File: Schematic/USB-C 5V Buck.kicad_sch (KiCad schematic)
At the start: 17 parts, among them Q25 CSD19531Q5A, Q26 CSD19531Q5A, U12 LM5148RGYR

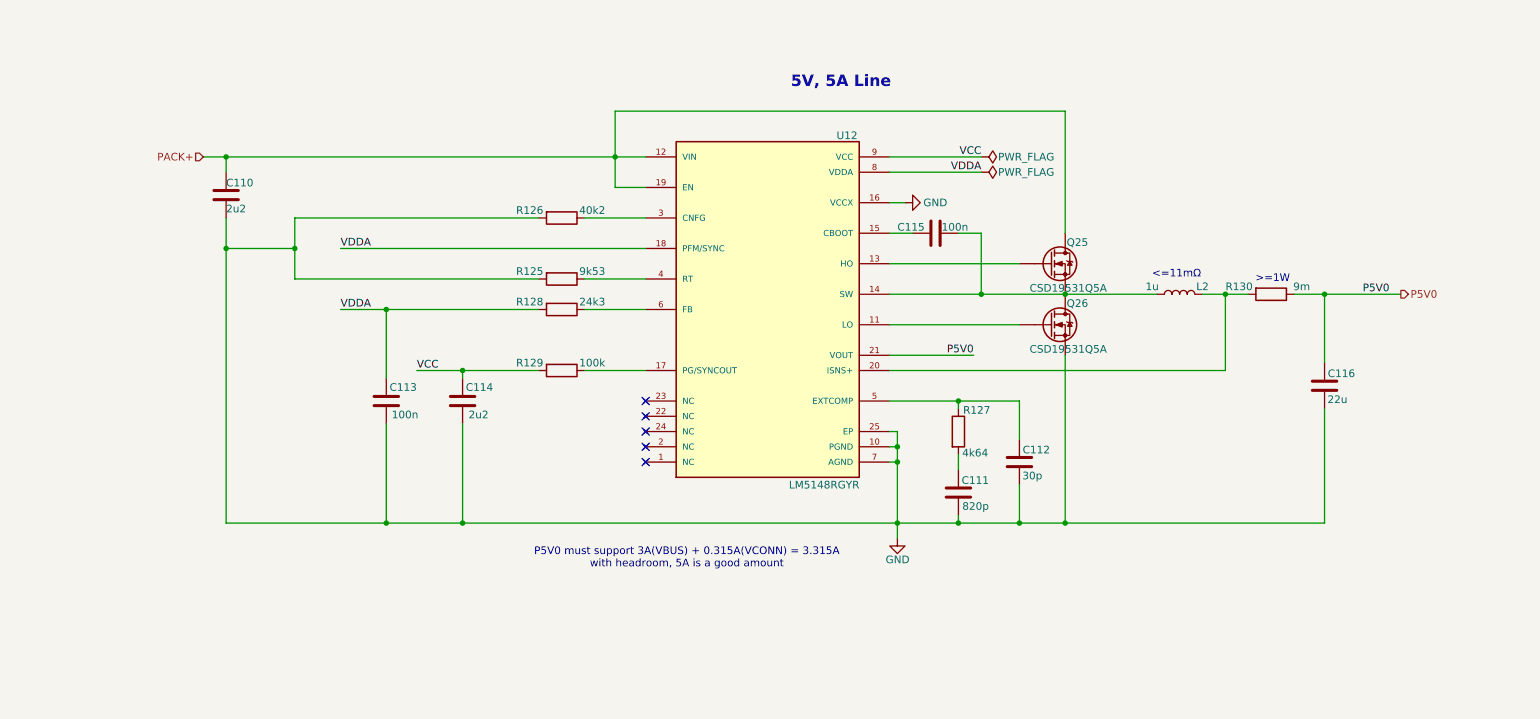
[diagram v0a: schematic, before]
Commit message: added sensors?
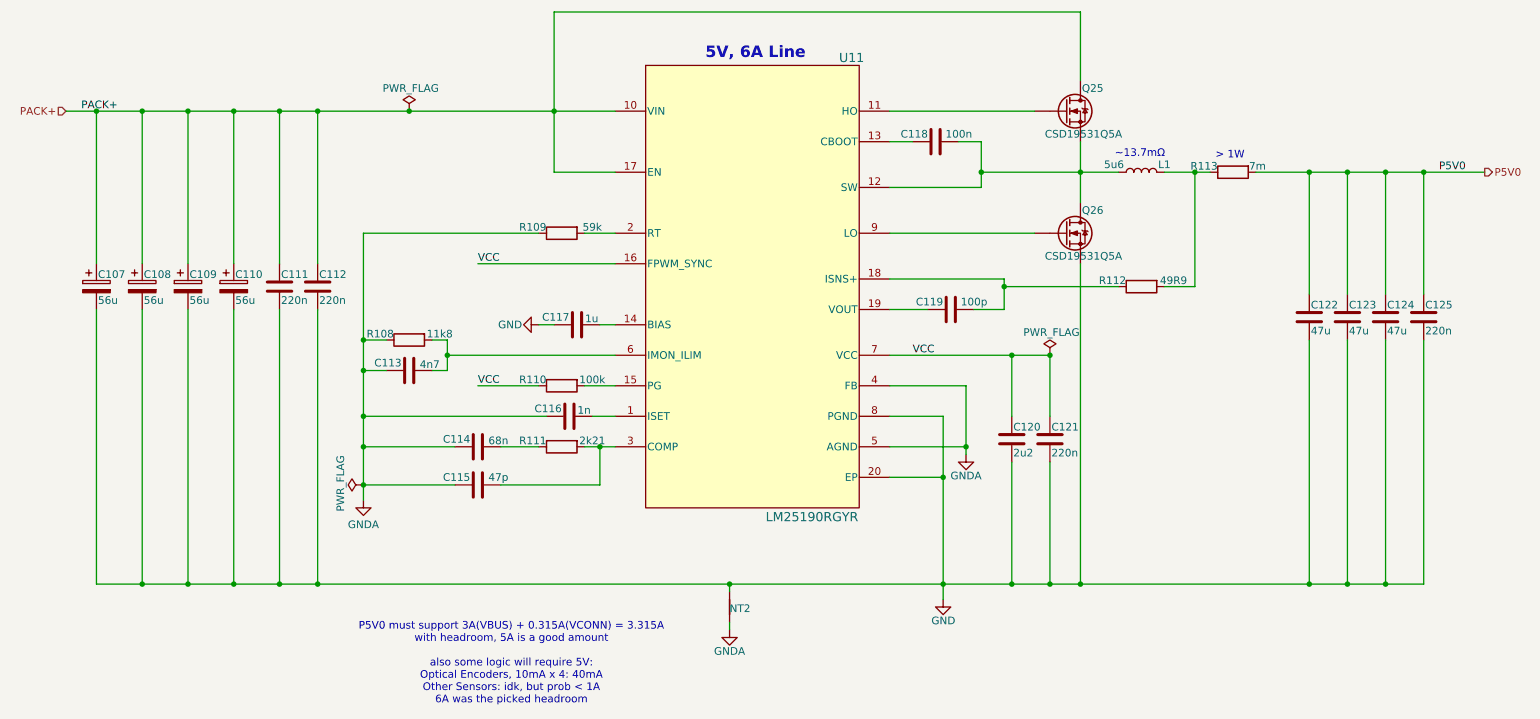
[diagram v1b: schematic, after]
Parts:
- removed C110: 2u2, symbol Device:C
- removed L2: 1u, symbol Device:L
- removed R125: 9k53, symbol Device:R
- removed R126: 40k2, symbol Device:R
- removed R127: 4k64, symbol Device:R
- removed R128: 24k3, symbol Device:R
- removed R129: 100k, symbol Device:R
- removed R130: 9m, symbol Device:R
- removed U12: LM5148RGYR, LM5148RGYR:QFN50P550X350X100-25N, symbol LM5148RGYR:LM5148RGYR
- added C107, C108, C109, C110: 56u, symbol Device:C_Polarized
- added C117: 1u, symbol Device:C
- added C118: 100n, symbol Device:C
- added C119: 100p, symbol Device:C
- added C120: 2u2, symbol Device:C
- added C121, C125: 220n, symbol Device:C
- added C122, C123, C124: 47u, symbol Device:C
- added L1: 5u6, symbol Device:L
- added NT2: NetTie_2, symbol Device:NetTie_2
- added R108: 11k8, symbol Device:R
- added R109: 59k, symbol Device:R
- added R110: 100k, symbol Device:R
- added R111: 2k21, symbol Device:R
- added R112: 49R9, symbol Device:R
- added R113: 7m, symbol Device:R
- added U11: LM25190RGYR, RGY0019C-MFG, symbol LM25190RGYR:LM25190RGYR
- C111: value 820p -> 220n
- C112: value 30p -> 220n
- C113: value 100n -> 4n7
- C114: value 2u2 -> 68n
- C115: value 100n -> 47p
- C116: value 22u -> 1n
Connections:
- net GND: now also C111.2, C112.2, C107.2, C108.2, C109.2, C110.2, C117.1, C120.2, C121.2, C122.2, C123.2, C124.2, C125.2, NT2.2, U11.20 (EP), U11.8 (PGND); no longer C111.1, C112.1, C113.2, C114.2, C116.1
- net P5V0: now also C122.1, C123.1, C124.1, C125.1, R113.2; no longer C116.2
- net PACK+: now also C111.1, C112.1, C107.1, C108.1, C109.1, C110.1, U11.10 (VIN), U11.17 (EN)
- net VCC: now also C120.1, C121.1, R110.1, U11.16 (FPWM_SYNC), U11.7 (VCC); no longer C114.1
- net at Q25.1 (S), Q25.2 (S), Q25.3 (S)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: now also C118.2, L1.1, U11.12 (SW); no longer C115.1
- net at C115.2: now also R111.2, U11.3 (COMP)
- net at Q26.4 (G): now also U11.9 (LO)
- net at Q25.4 (G): now also U11.11 (HO)
- net VDDA renamed GNDA
- net GNDA: now also C114.1, C115.1, C116.1, NT2.1, R108.1, R109.1, U11.4 (FB), U11.5 (AGND)
- new net: C118.1, U11.13 (CBOOT)
- new net: C114.2, R111.1
- new net: C116.2, U11.1 (ISET)
- new net: L1.2, R112.2, R113.1
- new net: C117.2, U11.14 (BIAS)
- new net: R110.2, U11.15 (PG)
- new net: C119.2, R112.1, U11.18 (ISNS+)
- new net: C119.1, U11.19 (VOUT)
- new net: R109.2, U11.2 (RT)
- new net: C113.2, R108.2, U11.6 (IMON_ILIM)
- no-connect marks 5 -> 0
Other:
- note added: "5V, 6A Line"
- note added: "> 1W"
- note added: "P5V0 must support 3A(VBUS) + 0.315A(VCONN) = 3.315A with headroom, 5A is a good amount also some logic will require 5V: Optical Encoders, 10mA x 4: 40mA Other Sensors: idk, but prob < 1A 6A was the picked headroom"
- note added: "~13.7mΩ"
- note removed: "5V, 5A Line"
- note removed: "<=11mΩ"
- note removed: ">=1W"
- note removed: "P5V0 must support 3A(VBUS) + 0.315A(VCONN) = 3.315A with headroom, 5A is a good amount"
